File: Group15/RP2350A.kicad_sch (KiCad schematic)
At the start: 3 parts, among them U1 RP2350A, U2 W25Q128JVS

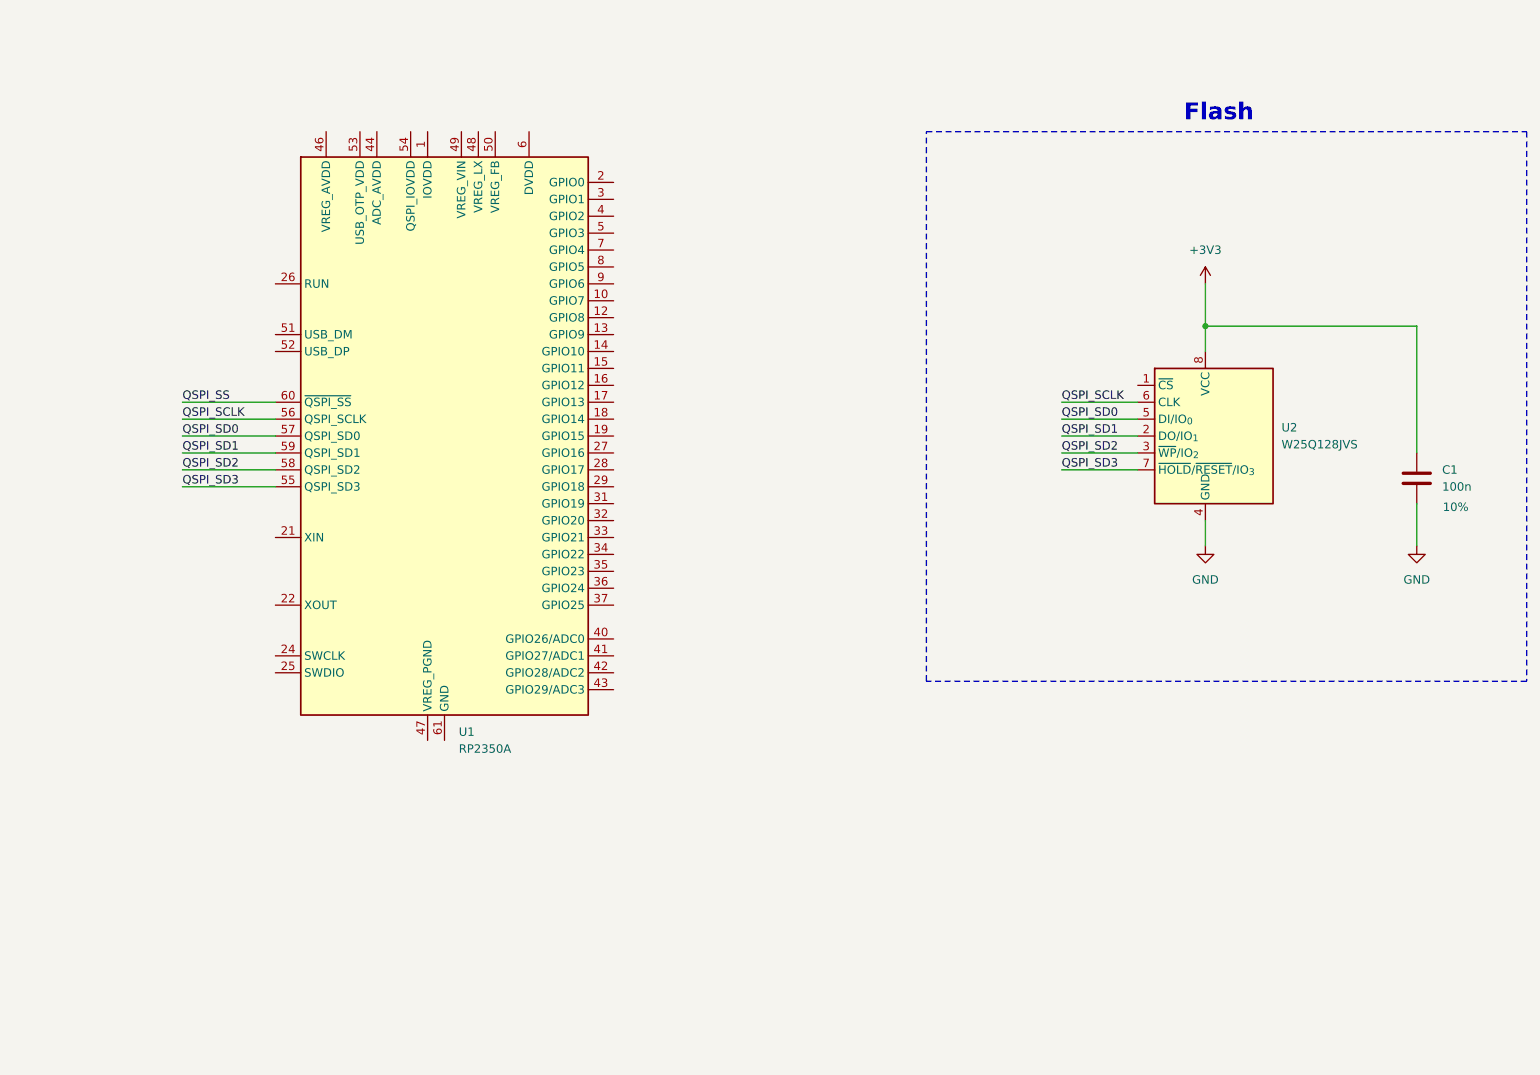
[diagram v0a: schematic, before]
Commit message: added board
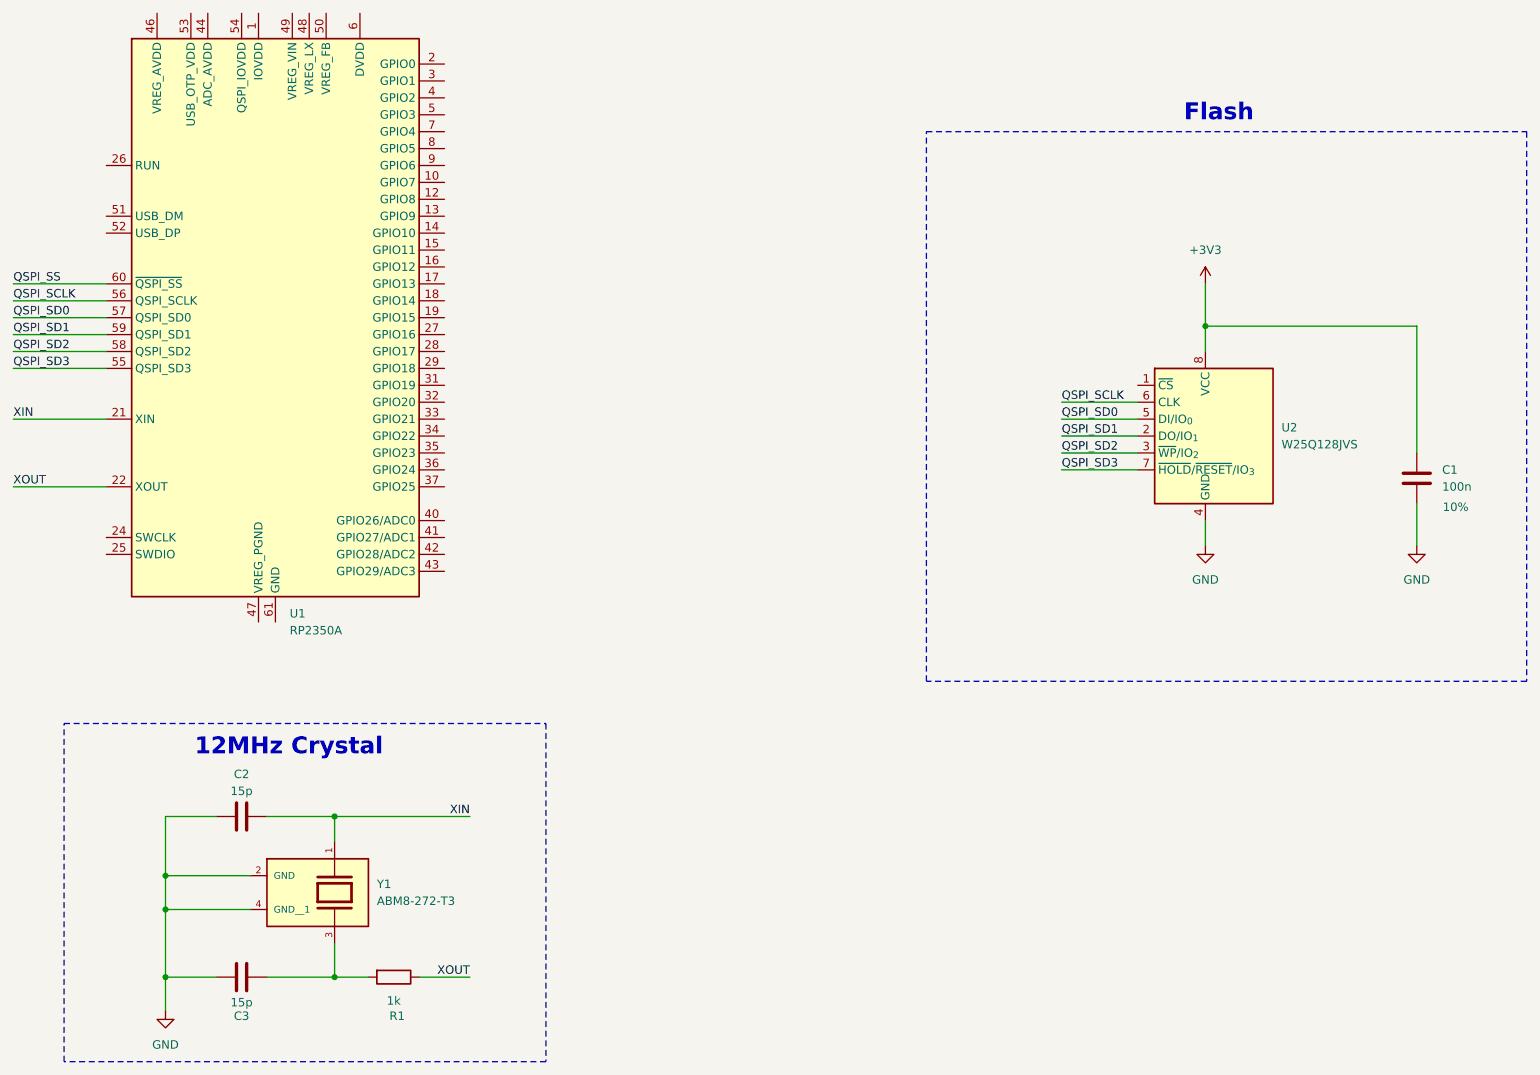
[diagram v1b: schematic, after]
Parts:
- added C2, C3: 15p, symbol Device:C
- added R1: 1k, symbol Device:R
- added Y1: ABM8-272-T3, Footprint_Library:XTAL_ABM8-272-T3, symbol Symbol_Library:ABM8-272-T3
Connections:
- net GND: now also C2.1, C3.1, Y1.2 (GND), Y1.4 (GND__1)
- net XIN: now reaches U1.21 (XIN)
- net XIN: now also C2.2, Y1.1
- net XOUT: now reaches U1.22 (XOUT)
- net XOUT: now also R1.1
- new net: C3.2, R1.2, Y1.3
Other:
- note added: "12MHz Crystal"
- moved on the sheet: U1
